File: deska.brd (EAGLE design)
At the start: 65.7 x 52.1 mm, 23 parts, among them Q1 BC547, X1 JST-XH-03-PIN-LONG-PAD, X2 JST-XH-03-PIN-LONG-PAD, X3 JST-XH-03-PIN-LONG-PAD, X4 JST-XH-04-PIN-LONG-PAD, X5 JST-XH-04-PIN-LONG-PAD, X6 JST-XH-04-PIN-LONG-PAD, X7 JST-XH-03-PIN-LONG-PAD

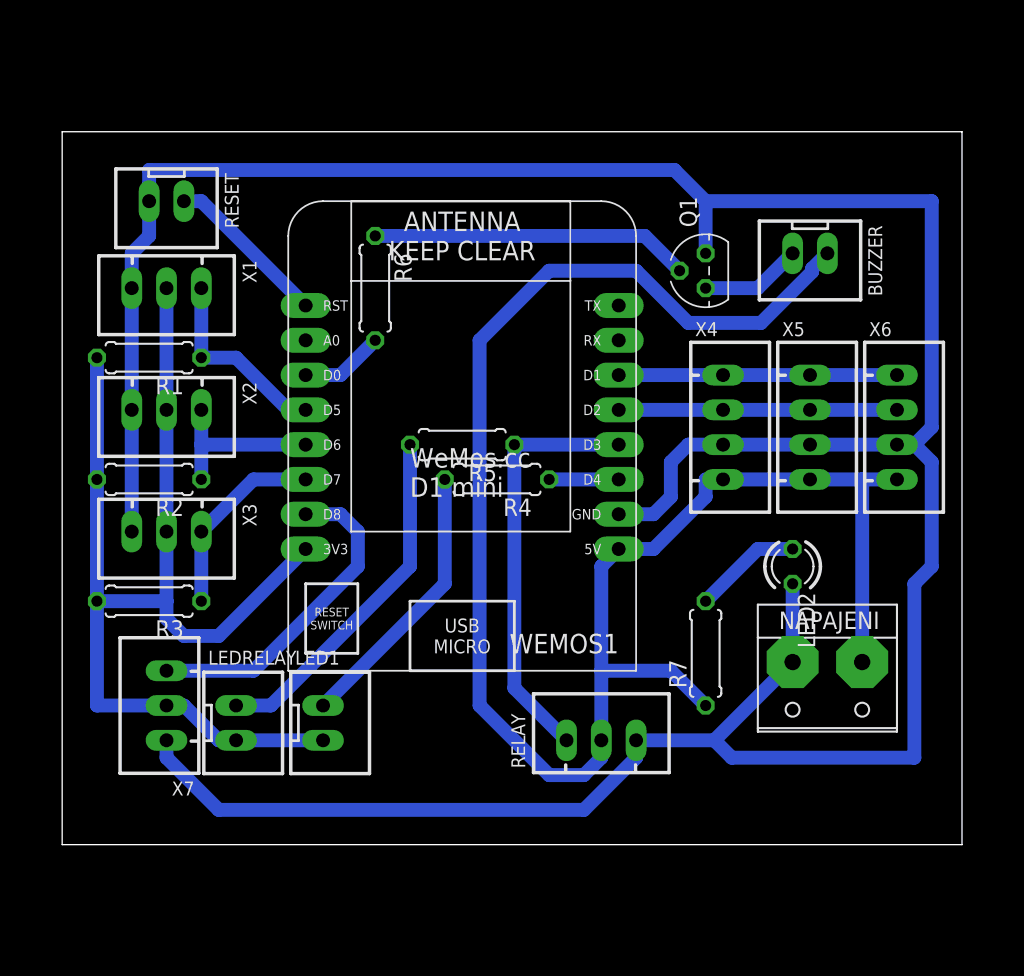
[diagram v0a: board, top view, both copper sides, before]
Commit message: +
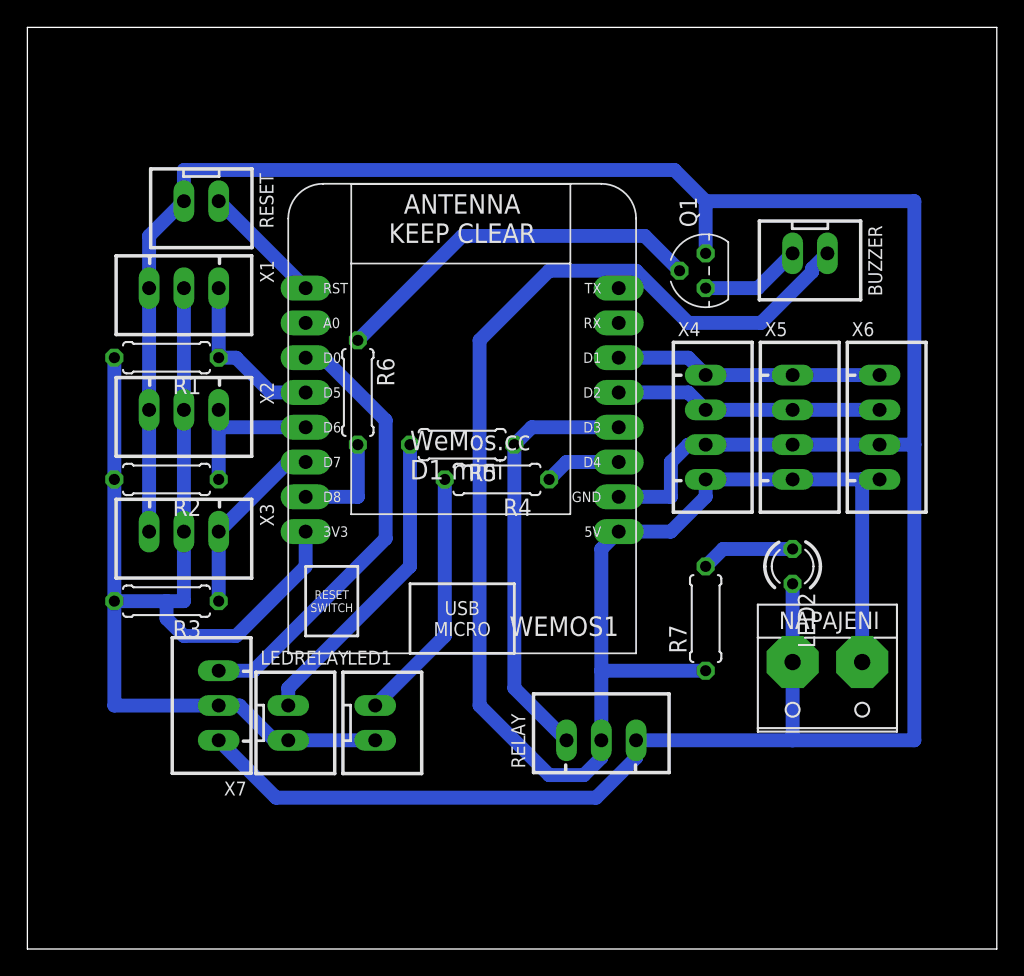
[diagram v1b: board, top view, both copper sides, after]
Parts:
- moved R6 7.73 mm to (38.1, 38.1)
- moved LEDRELAY 3.81 mm to (33.0, 14.0)
- moved X7 3.81 mm to (27.9, 15.2)
- moved LED1 3.81 mm to (39.4, 14.0)
- moved RESET 2.54 mm to (26.7, 52.1)
- moved R7 2.54 mm to (63.5, 21.6)
- moved X5 1.27 mm to (69.8, 35.6)
- moved WEMOS1 1.27 mm to (44.5, 38.1)
- moved R1 1.27 mm to (24.1, 40.6)
- moved R2 1.27 mm to (24.1, 31.8)
- moved R3 1.27 mm to (24.1, 22.9)
- moved X1 1.27 mm to (25.4, 45.7)
- moved X2 1.27 mm to (25.4, 36.8)
- moved X3 1.27 mm to (25.4, 27.9)
- moved X4 1.27 mm to (63.5, 35.6)
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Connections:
- removed net N$3: WEMOS1.D8, X7.3
- new net N$10: WEMOS1.D0, X7.3
- net N$8: now also WEMOS1.D8; no longer WEMOS1.D0
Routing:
- net N$10: track 0.00 -> 32.6 mm
- net N$3: track 24.0 -> 0.00 mm
- net GND: track 230.9 -> 216.0 mm
- net +3V3: track 85.5 -> 90.0 mm
- net N$7: track 23.3 -> 27.7 mm
- net N$5: track 12.0 -> 8.98 mm
- net N$2: track 25.8 -> 22.7 mm
- net N$1: track 14.3 -> 12.5 mm
- net N$6: track 20.2 -> 18.6 mm
- net +5V: track 130.5 -> 128.9 mm
- net N$8: track 6.13 -> 7.62 mm
- net N$19: track 12.7 -> 11.4 mm
- net N$4: track 7.93 -> 6.88 mm
- net N$9: track 14.3 -> 13.5 mm
- net N$12: track 20.3 -> 19.6 mm
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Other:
- board size 65.7 x 52.1 mm -> 70.8 x 67.3 mm
